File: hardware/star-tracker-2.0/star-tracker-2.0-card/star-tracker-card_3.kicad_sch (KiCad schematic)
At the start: 38 parts, among them J5 DM3BT-DSF-PEJS, U11 ICM-42688-P, U12 TCAN330, U13 EMMC+RESET+5.1-COMPATIBLE-BA, U7 OSD3358-512M-BSM

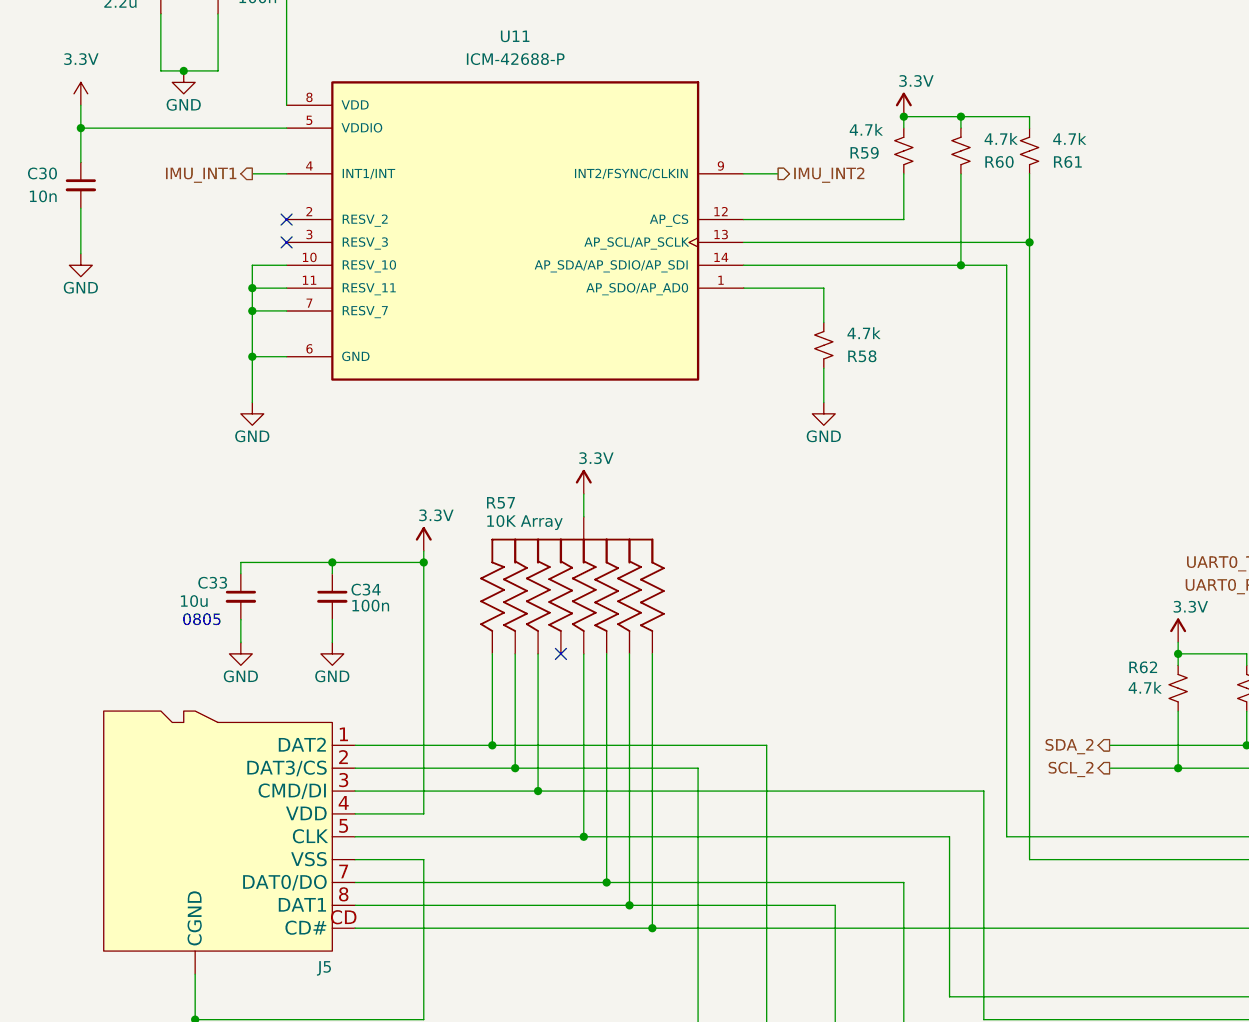
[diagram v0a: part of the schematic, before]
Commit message: Added extra Testpoints
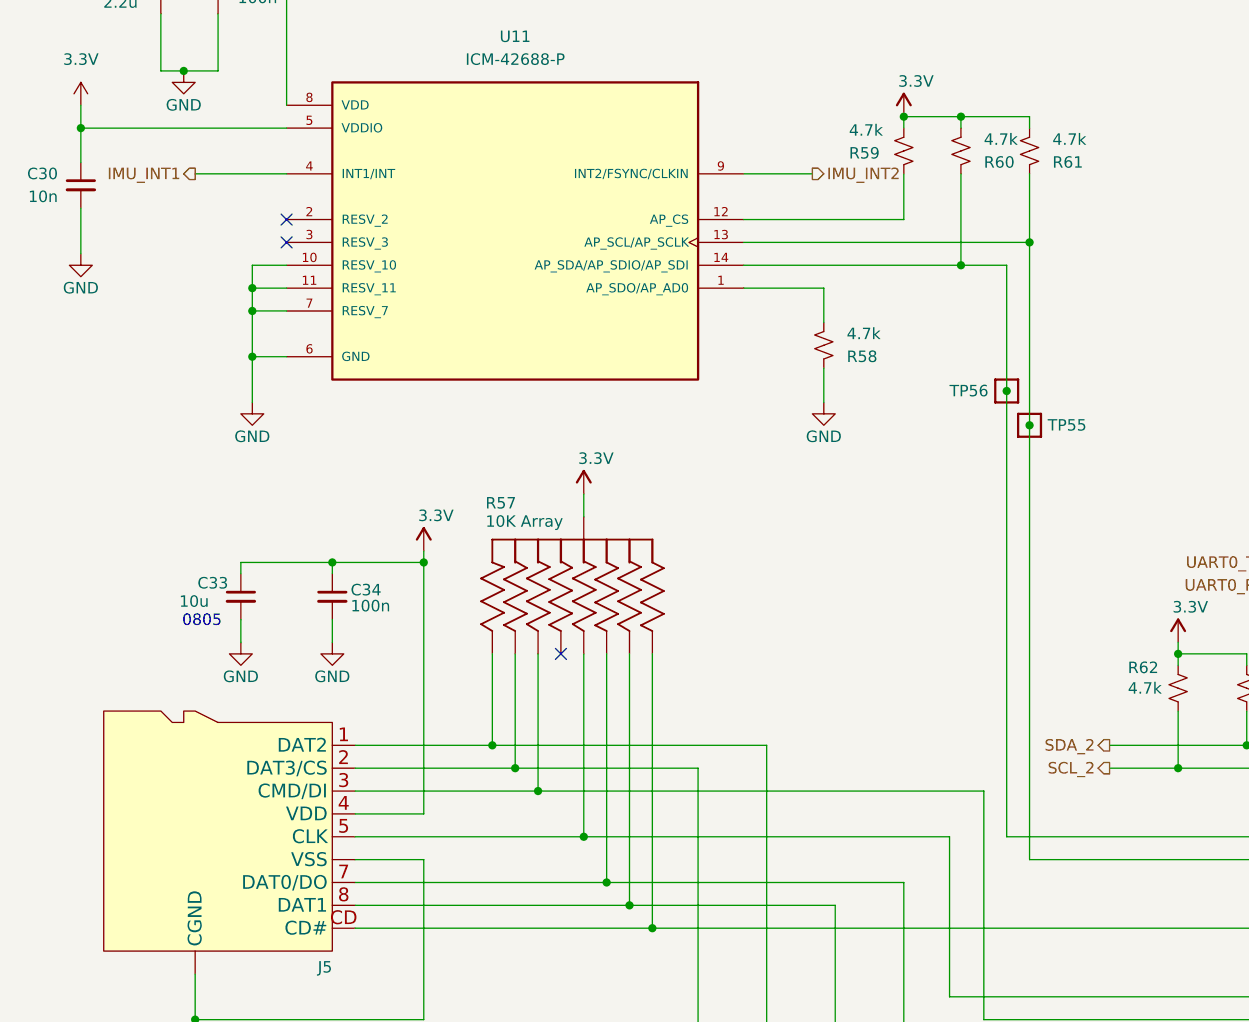
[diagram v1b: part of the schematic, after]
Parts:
- added TP55, TP56: Test-Point, oresat-misc:TestPoint_Pad_D1.0mm, symbol oresat-misc:Test-Point-1mm-round
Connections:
- net at R60.1, U11.14 (AP_SDA/AP_SDIO/AP_SDI), U7.A13 (SPI0_SCLK): now also TP56.1
- net at R61.1, U11.13 (AP_SCL/AP_SCLK), U7.B13 (SPI0_D0): now also TP55.1
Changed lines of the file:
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@@
 	)
 	(junction
+		(at 132.08 93.98)
+		(diameter 0)
+		(color 0 0 0 0)
+	)
+	(junction
 		(at 151.13 123.19)
 		(diameter 0)
@@
 	)
 	(junction
+		(at 134.62 97.79)
+		(diameter 0)
+		(color 0 0 0 0)
+	)
+	(junction
 		(at 292.1 179.07)
 		(diameter 0)
@@
 	(wire
 		(pts
+			(xy 132.08 93.98) (xy 132.08 80.01)
+		)
+		(stroke
+			(width 0.1524)
+			(type solid)
+		)
+	)
+	(wire
+		(pts
 			(xy 102.87 82.55) (xy 111.76 82.55)
 		)
@@
 	(wire
 		(pts
+			(xy 102.87 69.85) (xy 110.49 69.85)
+		)
+		(stroke
+			(width 0)
+			(type default)
+		)
+	)
+	(wire
+		(pts
 			(xy 158.75 123.19) (xy 158.75 124.46)
 		)
@@
 	(wire
 		(pts
+			(xy 41.91 69.85) (xy 52.07 69.85)
+		)
+		(stroke
+			(width 0)
+			(type default)
+		)
+	)
+	(wire
+		(pts
 			(xy 334.01 201.93) (xy 323.85 201.93)
 		)
@@
 	(wire
 		(pts
-			(xy 132.08 143.51) (xy 132.08 80.01)
+			(xy 132.08 143.51) (xy 132.08 93.98)
 		)
 		(stroke
@@
 	(wire
 		(pts
+			(xy 134.62 97.79) (xy 134.62 77.47)
+		)
+		(stroke
+			(width 0.1524)
+			(type solid)
+		)
+	)
+	(wire
+		(pts
 			(xy 400.05 153.67) (xy 400.05 148.59)
 		)
@@
 	(wire
 		(pts
-			(xy 106.68 69.85) (xy 102.87 69.85)
-		)
-		(stroke
-			(width 0)
-			(type default)
-		)
-	)
-	(wire
-		(pts
 			(xy 265.43 135.89) (xy 265.43 120.65)
 		)
@@
 	(wire
 		(pts
-			(xy 134.62 146.05) (xy 134.62 77.47)
+			(xy 134.62 146.05) (xy 134.62 97.79)
 		)
 		(stroke
@@
 	(wire
 		(pts
-			(xy 52.07 69.85) (xy 48.26 69.85)
-		)
-		(stroke
-			(width 0)
-			(type default)
-		)
-	)
-	(wire
-		(pts
 			(xy 384.81 166.37) (xy 384.81 161.29)
 		)
@@
 	(hierarchical_label "IMU_INT1"
 		(shape output)
-		(at 48.26 69.85 180)
+		(at 41.91 69.85 180)
 		(effects
 			(font
@@
 	(hierarchical_label "IMU_INT2"
 		(shape output)
-		(at 106.68 69.85 0)
+		(at 110.49 69.85 0)
 		(effects
 			(font
@@
 	)
 	(symbol
+		(lib_id "oresat-misc:Test-Point-1mm-round")
+		(at 134.62 97.79 0)
+		(mirror y)
+		(unit 1)
+		(body_style 1)
+		(exclude_from_sim yes)
+		(in_bom no)
+		(on_board yes)
+		(in_pos_files yes)
+		(dnp no)
+		(property "Reference" "TP55"
+			(at 140.97 97.79 0)
+			(show_name no)
+			(do_not_autoplace no)
+			(effects
+				(font
+					(size 1.27 1.27)
+				)
+				(justify left)
+			)
+		)
+		(property "Value" "Test-Point"
+			(at 134.62 95.25 0)
+			(hide yes)
+			(show_name no)
+			(do_not_autoplace no)
+			(effects
+				(font
+					(size 1.27 1.27)
+				)
+			)
+		)
+		(property "Footprint" "oresat-misc:TestPoint_Pad_D1.0mm"
+			(at 134.62 87.63 0)
+			(hide yes)
+			(show_name no)
+			(do_not_autoplace no)
+			(effects
+				(font
+					(size 1.27 1.27)
+				)
+			)
+		)
+		(property "Datasheet" ""
+			(at 134.62 97.79 0)
+			(hide yes)
+			(show_name no)
+			(do_not_autoplace no)
+			(effects
+				(font
+					(size 1.27 1.27)
+				)
+			)
+		)
+		(property "Description" "1mm round SMT test point"
+			(at 134.62 97.79 0)
+			(hide yes)
+			(show_name no)
+			(do_not_autoplace no)
+			(effects
+				(font
+					(size 1.27 1.27)
+				)
+			)
+		)
+		(pin "1"
+		)
+		(instances
+			(project "star-tracker-card"
+				(path "/324e9eb5-7420-4b7e-862c-cc20bb28618a/c38dcfbe-e8e3-410e-98db-09d235320446"
+					(reference "TP55")
+					(unit 1)
+				)
+			)
+		)
+	)
+	(symbol
 		(lib_id "Device:C_Small")
 		(at 369.57 156.21 0)
@@
 					(unit 1)
 				)
+			)
+		)
+	)
+	(symbol
+		(lib_id "oresat-misc:Test-Point-1mm-round")
+		(at 132.08 93.98 0)
+		(mirror x)
+		(unit 1)
+		(body_style 1)
+		(exclude_from_sim yes)
+		(in_bom no)
+		(on_board yes)
+		(in_pos_files yes)
+		(dnp no)
+		(property "Reference" "TP56"
+			(at 125.73 93.98 0)
+			(show_name no)
+			(do_not_autoplace no)
+			(effects
+				(font
+					(size 1.27 1.27)
+				)
+				(justify left)
+			)
+		)
+		(property "Value" "Test-Point"
+			(at 132.08 96.52 0)
+			(hide yes)
+			(show_name no)
+			(do_not_autoplace no)
+			(effects
+				(font
+					(size 1.27 1.27)
+				)
+			)
+		)
+		(property "Footprint" "oresat-misc:TestPoint_Pad_D1.0mm"
+			(at 132.08 104.14 0)
+			(hide yes)
+			(show_name no)
+			(do_not_autoplace no)
+			(effects
+				(font
+					(size 1.27 1.27)
+				)
+			)
+		)
+		(property "Datasheet" ""
+			(at 132.08 93.98 0)
+			(hide yes)
+			(show_name no)
+			(do_not_autoplace no)
+			(effects
+				(font
+					(size 1.27 1.27)
+				)
+			)
+		)
+		(property "Description" "1mm round SMT test point"
+			(at 132.08 93.98 0)
+			(hide yes)
+			(show_name no)
+			(do_not_autoplace no)
+			(effects
+				(font
+					(size 1.27 1.27)
+				)
+			)
+		)
+		(pin "1"
+		)
+		(instances
+			(project "star-tracker-card"
+				(path "/324e9eb5-7420-4b7e-862c-cc20bb28618a/c38dcfbe-e8e3-410e-98db-09d235320446"
+					(reference "TP56")
+					(unit 1)
+				)
